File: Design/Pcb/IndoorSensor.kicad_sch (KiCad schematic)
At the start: 17 parts, among them J1 Conn_01x04_Pin, J2 Conn_01x06_Pin, J3 Conn_01x04_Pin, U1 MH-Z19B, U3 WeMos_D1_mini, U4 module_bme280_alt

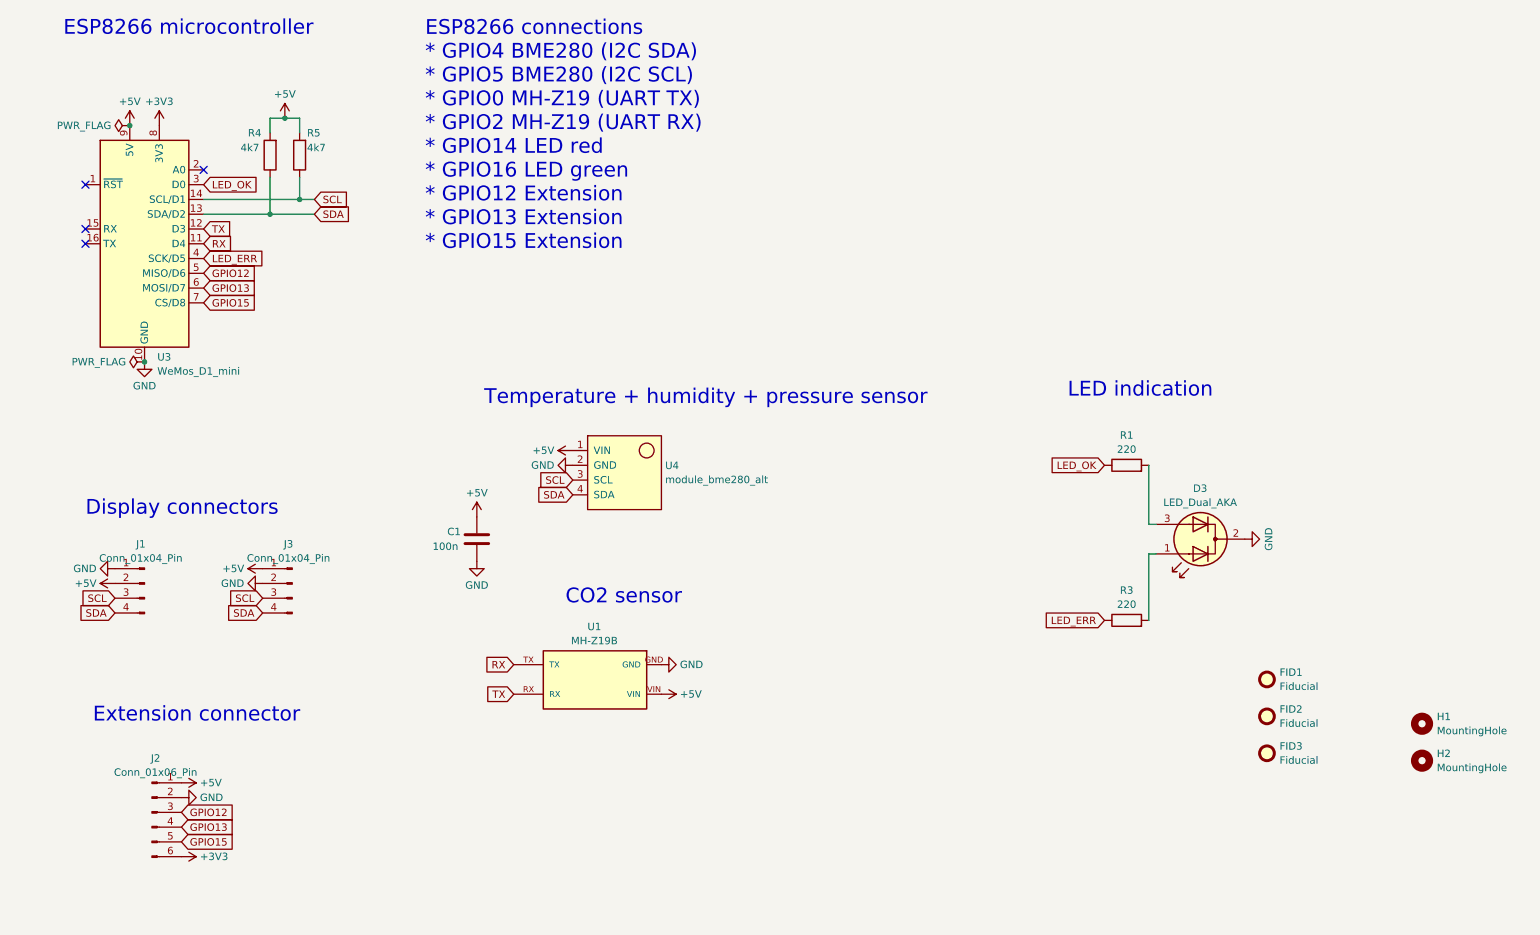
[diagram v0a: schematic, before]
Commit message: Add revision 2 design
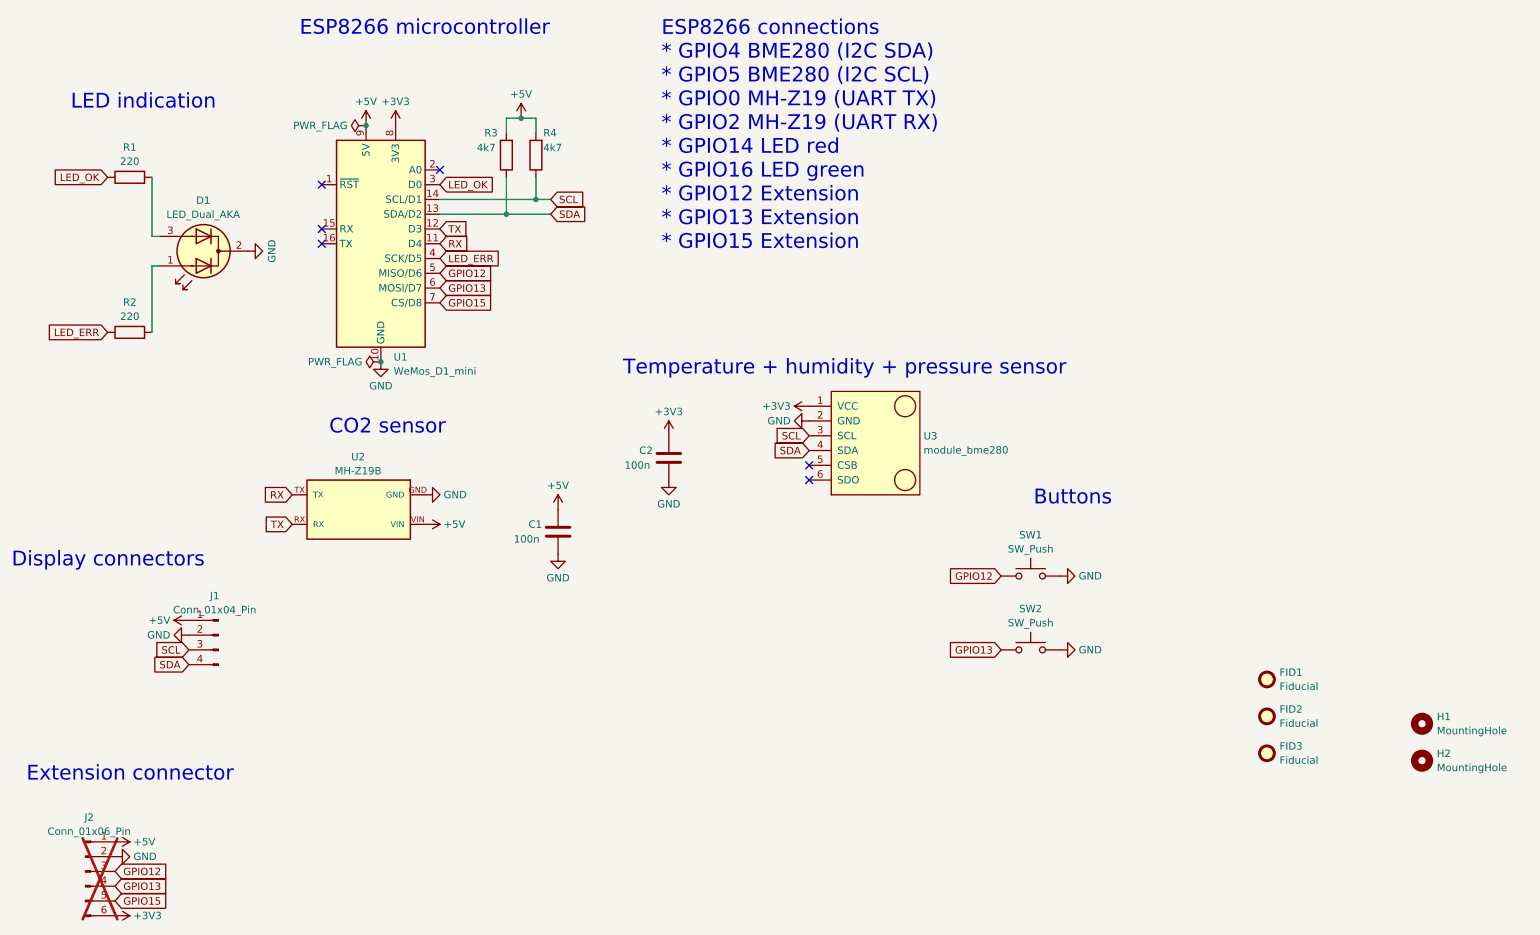
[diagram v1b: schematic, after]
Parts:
- removed J1: Conn_01x04_Pin, Connector_PinSocket_2.54mm:PinSocket_1x04_P2.54mm_Vertical, symbol Connector:Conn_01x04_Pin
- removed U4: module_bme280_alt, Libraries:module_bme280_alt, symbol usini_sensors:module_bme280_alt
- added C2: 100n, Capacitor_SMD:C_0805_2012Metric, symbol Device:C
- added SW1, SW2: SW_Push, Button_Switch_THT:SW_PUSH_6mm_H5mm, symbol Switch:SW_Push
- added U3: module_bme280, Libraries:module_bme280, symbol usini_sensors:module_bme280
- J2: footprint Connector_PinHeader_2.54mm:PinHeader_1x06_P2.54mm_Vertical -> Connector_PinSocket_2.54mm:PinSocket_1x06_P2.54mm_Vertical; now not fitted
- U1: renamed from U3; footprint Module:WEMOS_D1_mini_light -> RF_Module:WEMOS_D1_mini_light; symbol MCU_Module:WeMos_D1_mini -> RF_Module:WEMOS_D1_mini
- U2: renamed from U1; footprint MH-Z19B:MH-Z19B-FOOT -> Libraries:MH-Z19B-FOOT; Description_1 (none) -> Intelligent Infrared CO2 Module
- renumbered D3 to D1, J3 to J1, R3 to R2, R4 to R3, R5 to R4
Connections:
- net +3V3: now also C2.1, U3.1 (VCC)
- net GND: now also C2.2, SW1.2, SW2.2, U3.2 (GND)
- net GPIO12: now also SW1.1
- net GPIO13: now also SW2.1
- net SCL: now also U3.3 (SCL)
- net SDA: now also U3.4 (SDA)
- no-connect marks 4 -> 6
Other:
- note added: "Buttons"
- moved on the sheet: C1, D1, J1, R1, R2, R3, R4, U1, U2
